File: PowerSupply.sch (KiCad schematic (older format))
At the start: 28 parts

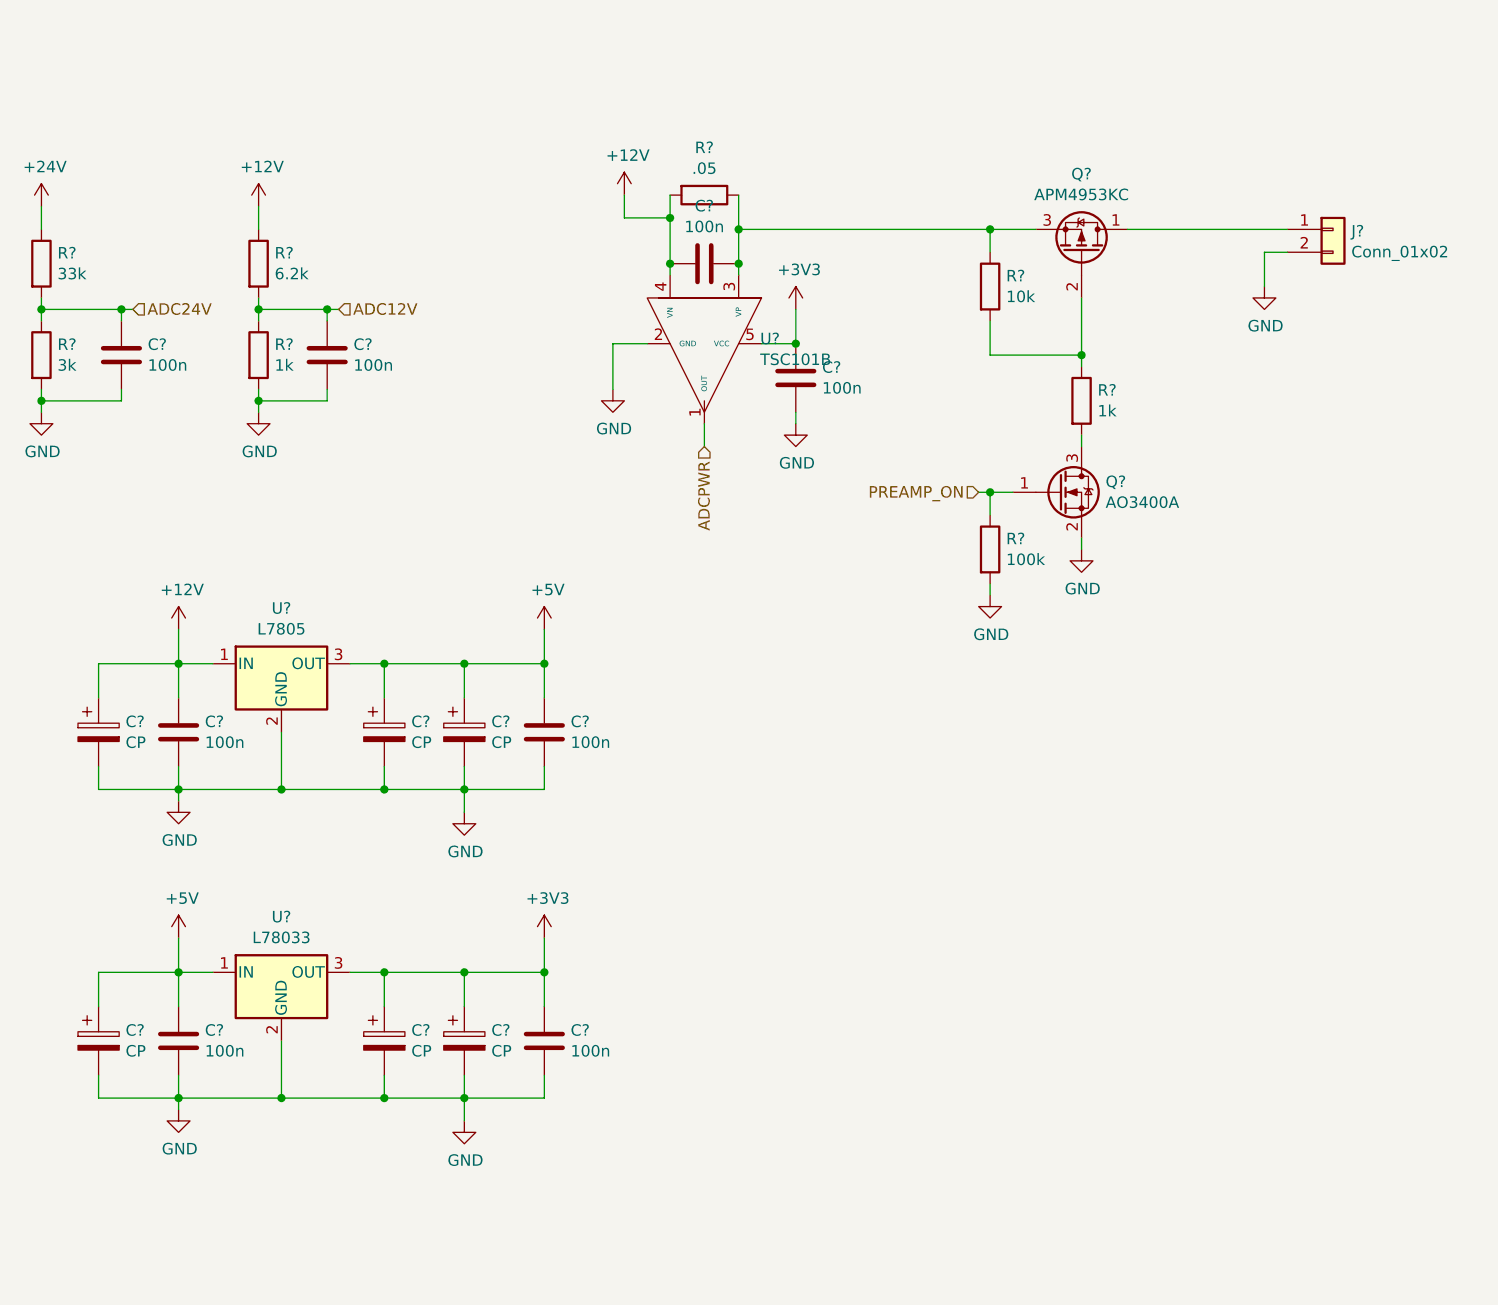
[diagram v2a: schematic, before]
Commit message: Ready for layout
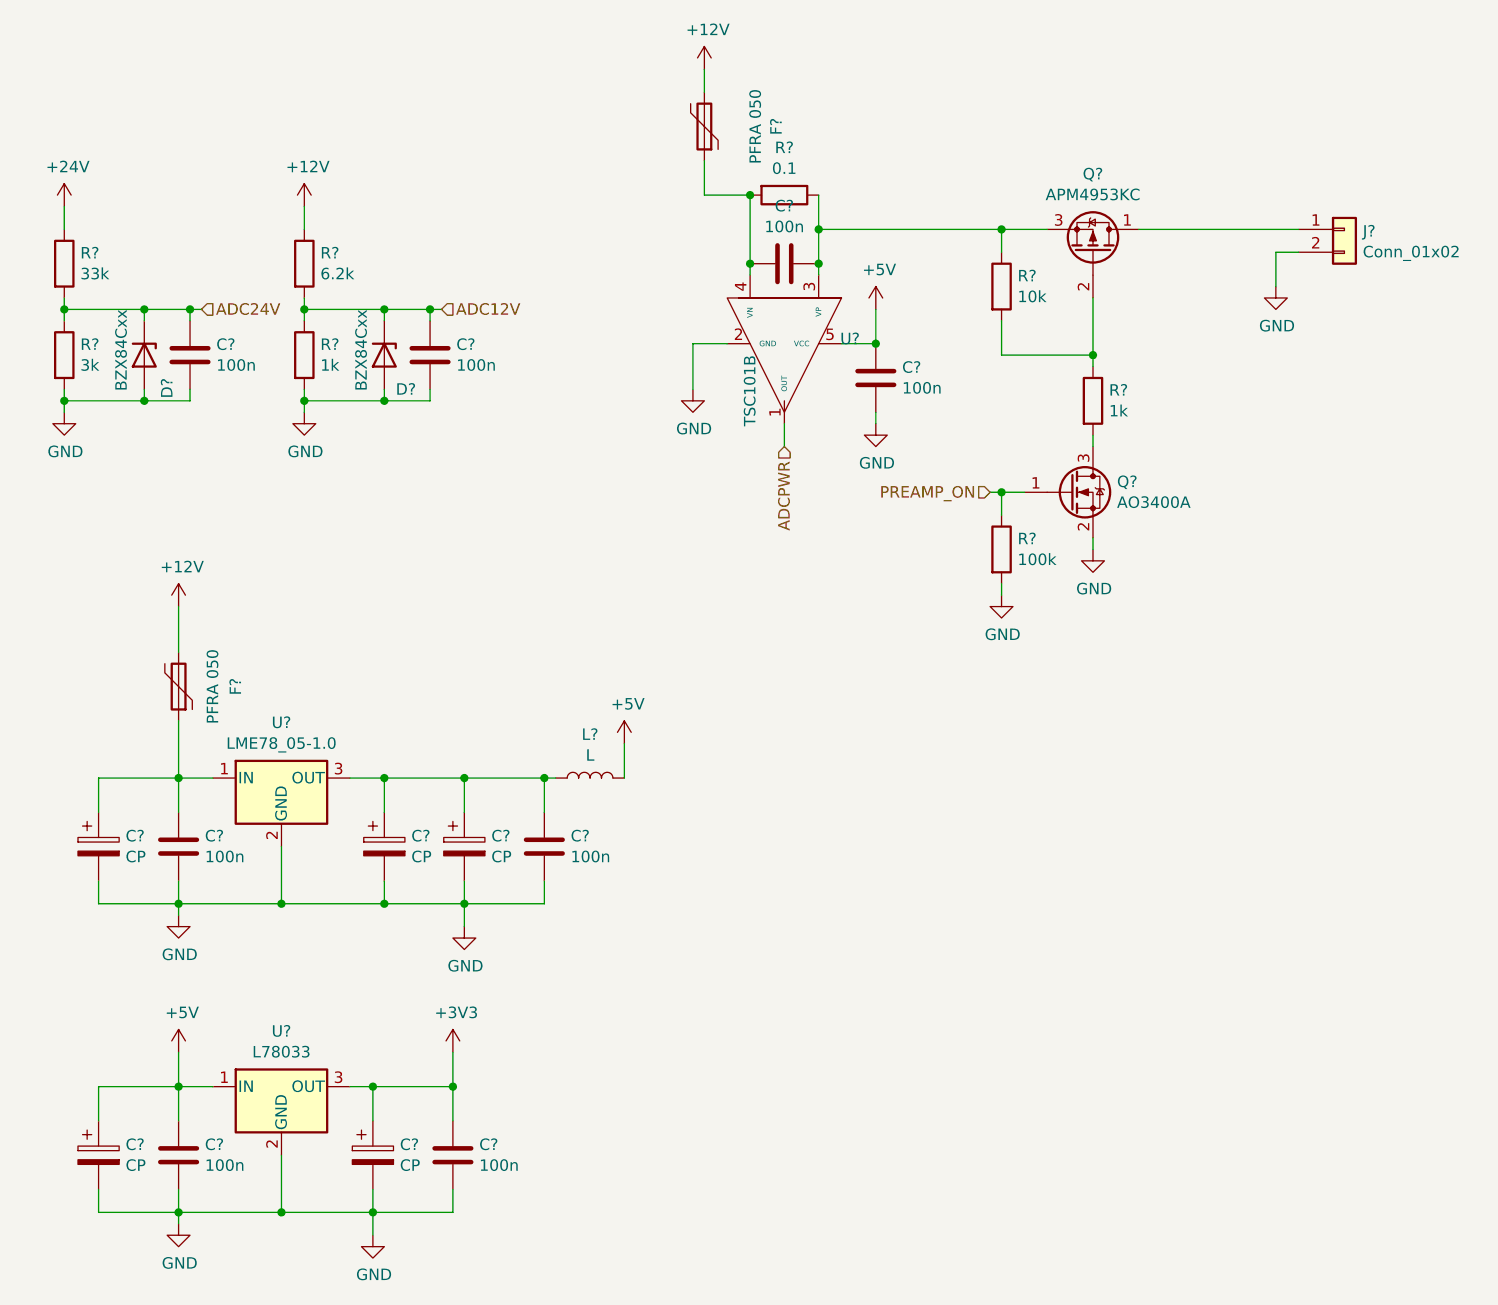
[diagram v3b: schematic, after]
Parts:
- removed C?: CP, symbol Device:CP
- added D? (x2): BZX84Cxx, Diode_SMD:D_SOT-23_ANK, symbol Diode:BZX84Cxx
- added F? (x2): PFRA 050, Fuse:Fuse_BelFuse_0ZRE0005FF_L8.3mm_W3.8mm, symbol Device:Polyfuse
- added L?: L, symbol Device:L
- R?: value .05 -> 0.1
- U?: value L7805 -> LME78_05-1.0; footprint (none) -> Package_TO_SOT_THT:TO-220-3_Vertical
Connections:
- net +12V: now also F?.2, F?.2; no longer C?.1, C?.1, C?.1, R?.2, U?.1 (IN), U?.4 (VN)
- net +3V3: no longer C?.1, U?.5 (VCC)
- net +5V: now also C?.1, U?.5 (VCC), L?.2; no longer C?.1, C?.1, C?.1, U?.3 (OUT)
- net ADC12V: now also D?.1 (K)
- net ADC24V: now also D?.1 (K)
- net GND: now also D?.2 (A), D?.2 (A)
- new net: C?.1, F?.1, R?.2, U?.4 (VN)
- new net: C?.1, C?.1, F?.1, U?.1 (IN)
- new net: C?.1, C?.1, C?.1, L?.1, U?.3 (OUT)
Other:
- moved on the sheet: C?, J?, Q?, R?, U?
